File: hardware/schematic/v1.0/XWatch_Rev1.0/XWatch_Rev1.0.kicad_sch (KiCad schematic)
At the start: 0 parts

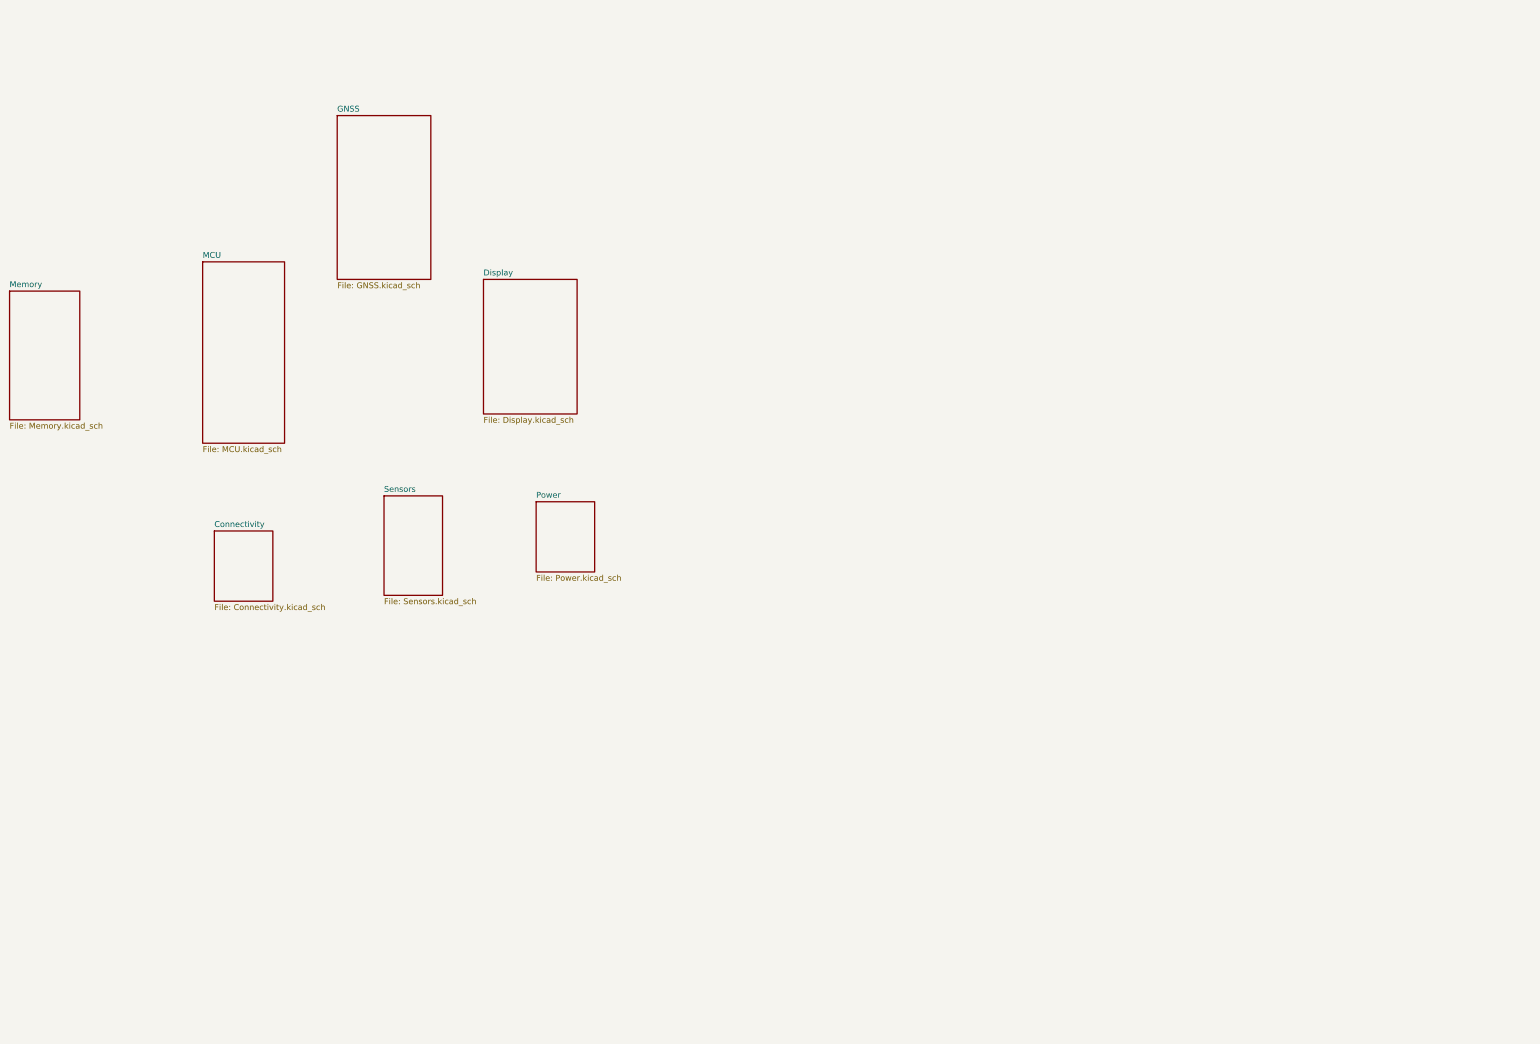
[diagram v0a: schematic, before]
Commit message: doc and sch update
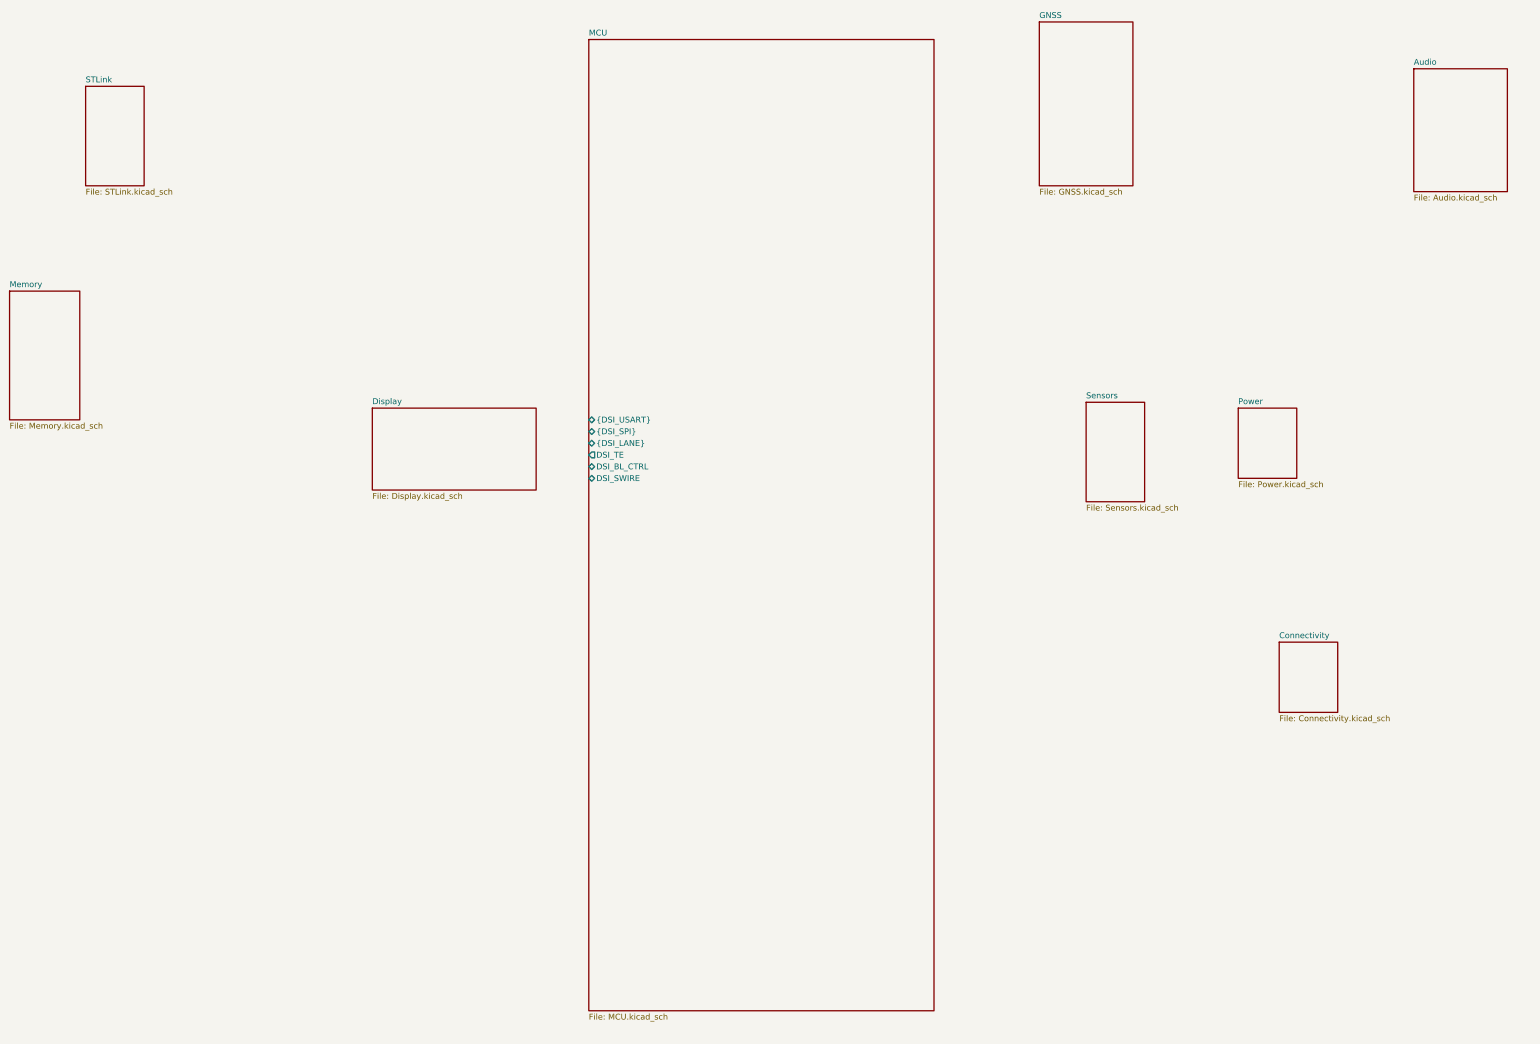
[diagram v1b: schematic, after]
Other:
- added sheet Audio (Audio.kicad_sch)
- added sheet STLink (STLink.kicad_sch)
- sheet MCU ports: added DSI_BL_CTRL, DSI_SWIRE, DSI_TE, {DSI_LANE}, {DSI_SPI}, {DSI_USART}; removed none
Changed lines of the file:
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@@
 	(generator "eeschema")
 	(generator_version "10.0")
-	(paper "A4")
+	(paper "A3")
 	(sheet
 		(at 63.5 101.6)
@@
 	)
 	(sheet
-		(at 134.62 63.5)
+		(at 287.02 43.18)
 		(size 20.32 35.56)
 		(exclude_from_sim no)
@@
 		)
 		(property "Sheetname" "GNSS"
-			(at 134.62 62.7884 0)
+			(at 287.02 42.4684 0)
 			(show_name no)
 			(do_not_autoplace no)
@@
 		)
 		(property "Sheetfile" "GNSS.kicad_sch"
-			(at 134.62 99.6446 0)
+			(at 287.02 79.3246 0)
 			(show_name no)
 			(do_not_autoplace no)
@@
 	)
 	(sheet
-		(at 144.78 146.05)
+		(at 297.18 125.73)
 		(size 12.7 21.59)
 		(exclude_from_sim no)
@@
 		)
 		(property "Sheetname" "Sensors"
-			(at 144.78 145.3384 0)
+			(at 297.18 125.0184 0)
 			(show_name no)
 			(do_not_autoplace no)
@@
 		)
 		(property "Sheetfile" "Sensors.kicad_sch"
-			(at 144.78 168.2246 0)
+			(at 297.18 147.9046 0)
 			(show_name no)
 			(do_not_autoplace no)
@@
 	)
 	(sheet
-		(at 177.8 147.32)
+		(at 330.2 127)
 		(size 12.7 15.24)
 		(exclude_from_sim no)
@@
 		)
 		(property "Sheetname" "Power"
-			(at 177.8 146.6084 0)
+			(at 330.2 126.2884 0)
 			(show_name no)
 			(do_not_autoplace no)
@@
 		)
 		(property "Sheetfile" "Power.kicad_sch"
-			(at 177.8 163.1446 0)
+			(at 330.2 142.8246 0)
 			(show_name no)
 			(do_not_autoplace no)
@@
 	)
 	(sheet
-		(at 107.95 153.67)
+		(at 339.09 177.8)
 		(size 12.7 15.24)
 		(exclude_from_sim no)
@@
 		)
 		(property "Sheetname" "Connectivity"
-			(at 107.95 152.9584 0)
+			(at 339.09 177.0884 0)
 			(show_name no)
 			(do_not_autoplace no)
@@
 		)
 		(property "Sheetfile" "Connectivity.kicad_sch"
-			(at 107.95 169.4946 0)
+			(at 339.09 193.6246 0)
 			(show_name no)
 			(do_not_autoplace no)
@@
 	)
 	(sheet
-		(at 166.37 99.06)
-		(size 20.32 29.21)
+		(at 142.24 127)
+		(size 35.56 17.78)
 		(exclude_from_sim no)
 		(in_bom yes)
@@
 		)
 		(property "Sheetname" "Display"
-			(at 166.37 98.3484 0)
+			(at 142.24 126.2884 0)
 			(show_name no)
 			(do_not_autoplace no)
@@
 		)
 		(property "Sheetfile" "Display.kicad_sch"
-			(at 166.37 128.8546 0)
+			(at 142.24 145.3646 0)
 			(show_name no)
 			(do_not_autoplace no)
@@
 	)
 	(sheet
-		(at 105.41 95.25)
-		(size 17.78 39.37)
+		(at 80.01 57.15)
+		(size 12.7 21.59)
+		(exclude_from_sim no)
+		(in_bom yes)
+		(on_board yes)
+		(dnp no)
+		(fields_autoplaced yes)
+		(stroke
+			(width 0.1524)
+			(type solid)
+		)
+		(fill
+			(color 0 0 0 0)
+		)
+		(property "Sheetname" "STLink"
+			(at 80.01 56.4384 0)
+			(show_name no)
+			(do_not_autoplace no)
+			(effects
+				(font
+					(size 1.27 1.27)
+				)
+				(justify left bottom)
+			)
+		)
+		(property "Sheetfile" "STLink.kicad_sch"
+			(at 80.01 79.3246 0)
+			(show_name no)
+			(do_not_autoplace no)
+			(effects
+				(font
+					(size 1.27 1.27)
+				)
+				(justify left top)
+			)
+		)
+		(instances
+			(project "XWatch_Rev1.0"
+				(path "/2e5e9480-7d2e-4148-a9bf-0ac7d46b20bc"
+					(page "10")
+				)
+			)
+		)
+	)
+	(sheet
+		(at 368.3 53.34)
+		(size 20.32 26.67)
+		(exclude_from_sim no)
+		(in_bom yes)
+		(on_board yes)
+		(dnp no)
+		(fields_autoplaced yes)
+		(stroke
+			(width 0.1524)
+			(type solid)
+		)
+		(fill
+			(color 0 0 0 0)
+		)
+		(property "Sheetname" "Audio"
+			(at 368.3 52.6284 0)
+			(show_name no)
+			(do_not_autoplace no)
+			(effects
+				(font
+					(size 1.27 1.27)
+				)
+				(justify left bottom)
+			)
+		)
+		(property "Sheetfile" "Audio.kicad_sch"
+			(at 368.3 80.5946 0)
+			(show_name no)
+			(do_not_autoplace no)
+			(effects
+				(font
+					(size 1.27 1.27)
+				)
+				(justify left top)
+			)
+		)
+		(instances
+			(project "XWatch_Rev1.0"
+				(path "/2e5e9480-7d2e-4148-a9bf-0ac7d46b20bc"
+					(page "9")
+				)
+			)
+		)
+	)
+	(sheet
+		(at 189.23 46.99)
+		(size 74.93 210.82)
 		(exclude_from_sim no)
 		(in_bom yes)
@@
 		)
 		(property "Sheetname" "MCU"
-			(at 105.41 94.5384 0)
+			(at 189.23 46.2784 0)
 			(show_name no)
 			(do_not_autoplace no)
@@
 		)
 		(property "Sheetfile" "MCU.kicad_sch"
-			(at 105.41 135.2046 0)
-			(show_name no)
-			(do_not_autoplace no)
-			(effects
-				(font
-					(size 1.27 1.27)
-				)
-				(justify left top)
-			)
-		)
+			(at 189.23 258.3946 0)
+			(show_name no)
+			(do_not_autoplace no)
+			(effects
+				(font
+					(size 1.27 1.27)
+				)
+				(justify left top)
+			)
+		)
+		(pin "{DSI_SPI}" bidirectional
+			(at 189.23 132.08 180)
+			(effects
+				(font
+					(size 1.27 1.27)
+				)
+				(justify left)
+			)
+		)
+		(pin "{DSI_USART}" bidirectional
+			(at 189.23 129.54 180)
+			(effects
+				(font
+					(size 1.27 1.27)
+				)
+				(justify left)
+			)
+		)
+		(pin "{DSI_LANE}" bidirectional
+			(at 189.23 134.62 180)
+			(effects
+				(font
+					(size 1.27 1.27)
+				)
+				(justify left)
+			)
+		)
+		(pin "DSI_TE" output
+			(at 189.23 137.16 180)
+			(effects
+				(font
+					(size 1.27 1.27)
+				)
+				(justify left)
+			)
+		)
+		(pin "DSI_BL_CTRL" bidirectional
+			(at 189.23 139.7 180)
+			(effects
+				(font
+					(size 1.27 1.27)
+				)
+				(justify left)
+			)
+		)
+		(pin "DSI_SWIRE" bidirectional
+			(at 189.23 142.24 180)
+			(effects
+				(font
+					(size 1.27 1.27)
+				)
+				(justify left)
+			)
+		)

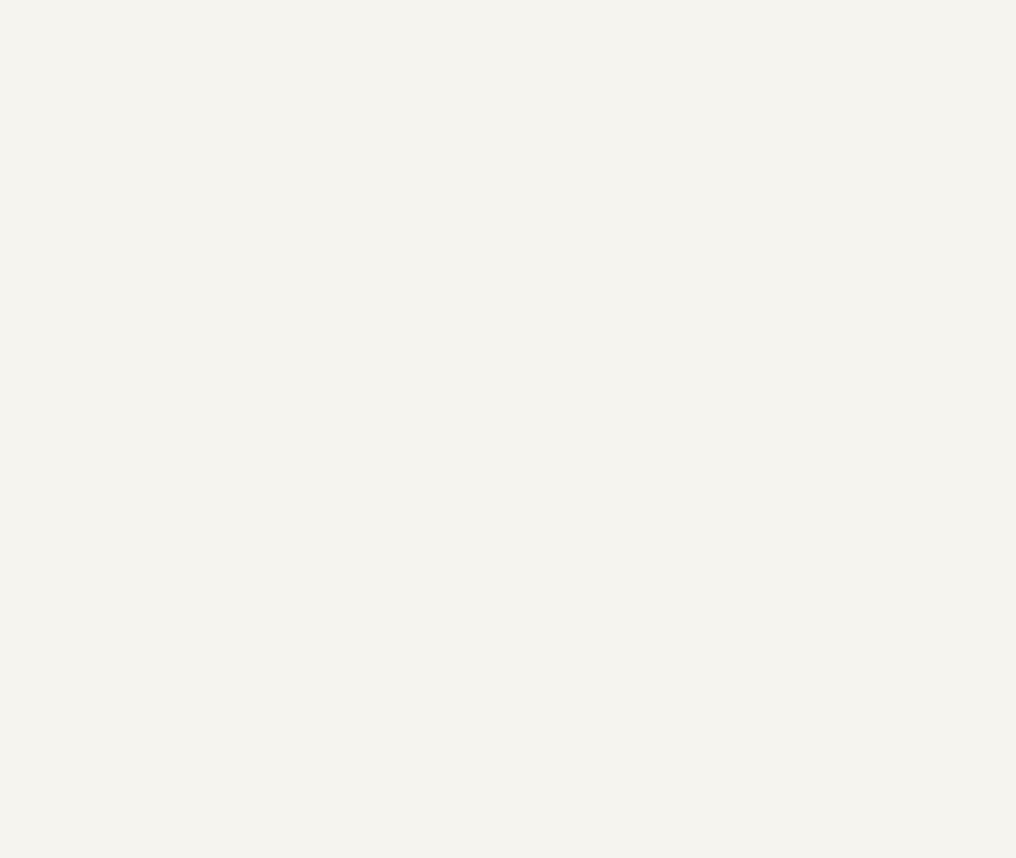
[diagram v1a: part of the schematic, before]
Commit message: doc and sch update
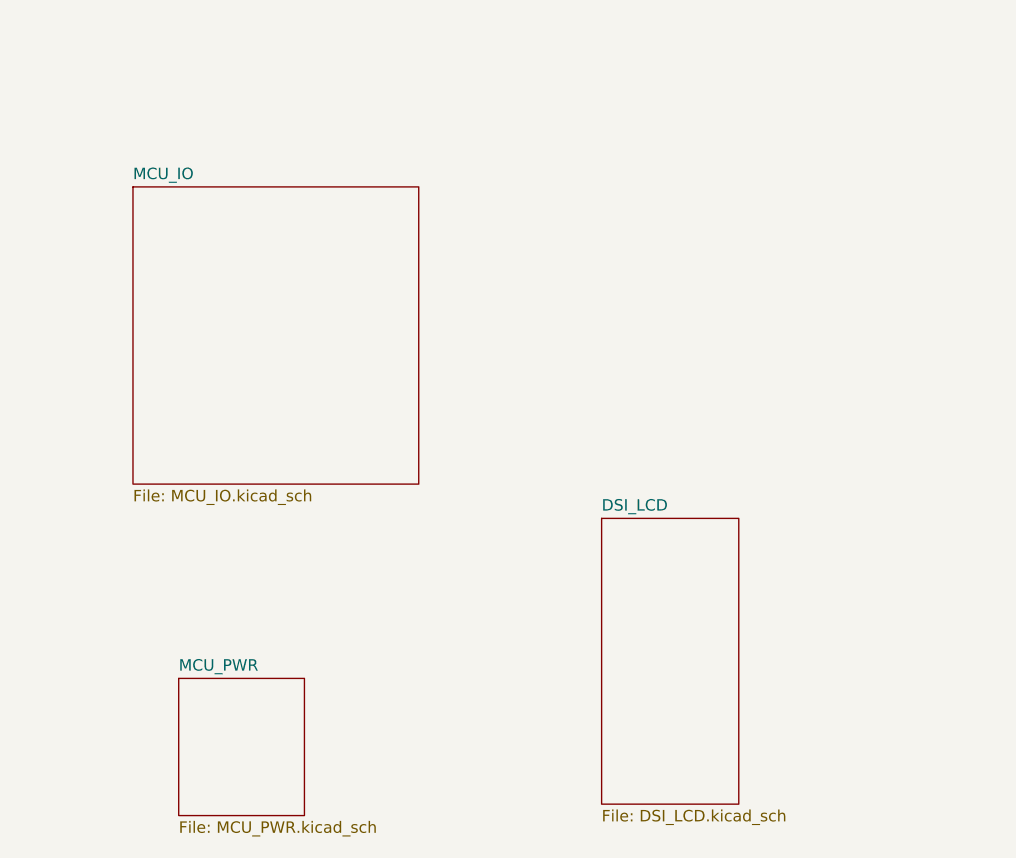
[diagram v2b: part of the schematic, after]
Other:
- added sheet DSI_LCD (DSI_LCD.kicad_sch)
- added sheet MCU_IO (MCU_IO.kicad_sch)
- added sheet MCU_PWR (MCU_PWR.kicad_sch)
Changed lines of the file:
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@@
+	)
+	(sheet
+		(at 81.28 245.11)
+		(size 13.97 15.24)
+		(exclude_from_sim no)
+		(in_bom yes)
+		(on_board yes)
+		(dnp no)
+		(fields_autoplaced yes)
+		(stroke
+			(width 0.1524)
+			(type solid)
+		)
+		(fill
+			(color 0 0 0 0)
+		)
+		(property "Sheetname" "MCU_PWR"
+			(at 81.28 244.3984 0)
+			(show_name no)
+			(do_not_autoplace no)
+			(effects
+				(font
+					(size 1.27 1.27)
+				)
+				(justify left bottom)
+			)
+		)
+		(property "Sheetfile" "MCU_PWR.kicad_sch"
+			(at 81.28 260.9346 0)
+			(show_name no)
+			(do_not_autoplace no)
+			(effects
+				(font
+					(size 1.27 1.27)
+				)
+				(justify left top)
+			)
+		)
+		(instances
+			(project "XWatch_Rev1.0"
+				(path "/2e5e9480-7d2e-4148-a9bf-0ac7d46b20bc"
+					(page "13")
+				)
+			)
+		)
+	)
+	(sheet
+		(at 128.27 227.33)
+		(size 15.24 31.75)
+		(exclude_from_sim no)
+		(in_bom yes)
+		(on_board yes)
+		(dnp no)
+		(fields_autoplaced yes)
+		(stroke
+			(width 0.1524)
+			(type solid)
+		)
+		(fill
+			(color 0 0 0 0)
+		)
+		(property "Sheetname" "DSI_LCD"
+			(at 128.27 226.6184 0)
+			(show_name no)
+			(do_not_autoplace no)
+			(effects
+				(font
+					(size 1.27 1.27)
+				)
+				(justify left bottom)
+			)
+		)
+		(property "Sheetfile" "DSI_LCD.kicad_sch"
+			(at 128.27 259.6646 0)
+			(show_name no)
+			(do_not_autoplace no)
+			(effects
+				(font
+					(size 1.27 1.27)
+				)
+				(justify left top)
+			)
+		)
+		(instances
+			(project "XWatch_Rev1.0"
+				(path "/2e5e9480-7d2e-4148-a9bf-0ac7d46b20bc"
+					(page "12")
+				)
+			)
+		)
 	)
 	(sheet
@@
 				)
 			)
+		)
+	)
+	(sheet
+		(at 76.2 190.5)
+		(size 31.75 33.02)
+		(exclude_from_sim no)
+		(in_bom yes)
+		(on_board yes)
+		(dnp no)
+		(fields_autoplaced yes)
+		(stroke
+			(width 0.1524)
+			(type solid)
+		)
+		(fill
+			(color 0 0 0 0)
+		)
+		(property "Sheetname" "MCU_IO"
+			(at 76.2 189.7884 0)
+			(show_name no)
+			(do_not_autoplace no)
+			(effects
+				(font
+					(size 1.27 1.27)
+				)
+				(justify left bottom)
+			)
+		)
+		(property "Sheetfile" "MCU_IO.kicad_sch"
+			(at 76.2 224.1046 0)
+			(show_name no)
+			(do_not_autoplace no)
+			(effects
+				(font
+					(size 1.27 1.27)
+				)
+				(justify left top)
+			)
+		)
+		(instances
+			(project "XWatch_Rev1.0"
+				(path "/2e5e9480-7d2e-4148-a9bf-0ac7d46b20bc"
+					(page "11")
+				)
+			)

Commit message: add rev2.0
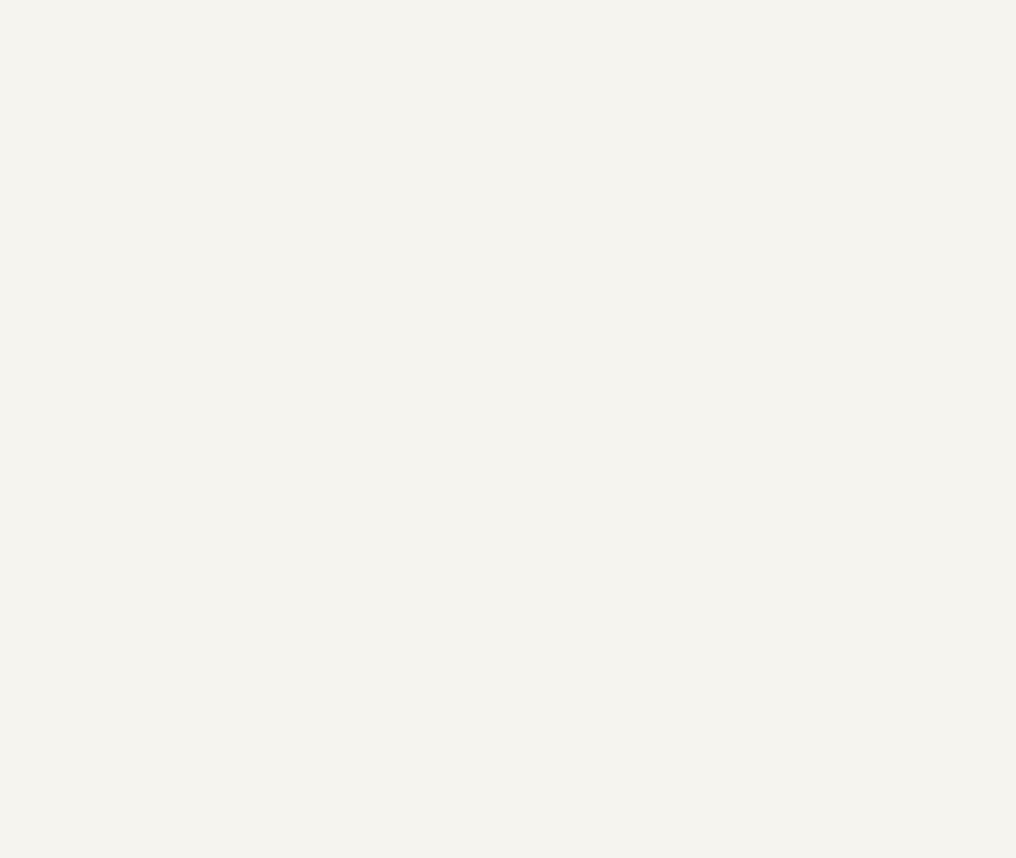
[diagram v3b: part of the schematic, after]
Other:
- removed sheet DSI_LCD
- removed sheet MCU_IO
- removed sheet MCU_PWR
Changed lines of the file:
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@@
-	)
-	(sheet
-		(at 81.28 245.11)
-		(size 13.97 15.24)
-		(exclude_from_sim no)
-		(in_bom yes)
-		(on_board yes)
-		(dnp no)
-		(fields_autoplaced yes)
-		(stroke
-			(width 0.1524)
-			(type solid)
-		)
-		(fill
-			(color 0 0 0 0)
-		)
-		(property "Sheetname" "MCU_PWR"
-			(at 81.28 244.3984 0)
-			(show_name no)
-			(do_not_autoplace no)
-			(effects
-				(font
-					(size 1.27 1.27)
-				)
-				(justify left bottom)
-			)
-		)
-		(property "Sheetfile" "MCU_PWR.kicad_sch"
-			(at 81.28 260.9346 0)
-			(show_name no)
-			(do_not_autoplace no)
-			(effects
-				(font
-					(size 1.27 1.27)
-				)
-				(justify left top)
-			)
-		)
-		(instances
-			(project "XWatch_Rev1.0"
-				(path "/2e5e9480-7d2e-4148-a9bf-0ac7d46b20bc"
-					(page "13")
-				)
-			)
-		)
-	)
-	(sheet
-		(at 128.27 227.33)
-		(size 15.24 31.75)
-		(exclude_from_sim no)
-		(in_bom yes)
-		(on_board yes)
-		(dnp no)
-		(fields_autoplaced yes)
-		(stroke
-			(width 0.1524)
-			(type solid)
-		)
-		(fill
-			(color 0 0 0 0)
-		)
-		(property "Sheetname" "DSI_LCD"
-			(at 128.27 226.6184 0)
-			(show_name no)
-			(do_not_autoplace no)
-			(effects
-				(font
-					(size 1.27 1.27)
-				)
-				(justify left bottom)
-			)
-		)
-		(property "Sheetfile" "DSI_LCD.kicad_sch"
-			(at 128.27 259.6646 0)
-			(show_name no)
-			(do_not_autoplace no)
-			(effects
-				(font
-					(size 1.27 1.27)
-				)
-				(justify left top)
-			)
-		)
-		(instances
-			(project "XWatch_Rev1.0"
-				(path "/2e5e9480-7d2e-4148-a9bf-0ac7d46b20bc"
-					(page "12")
-				)
-			)
-		)
 	)
 	(sheet
@@
 				)
 			)
-		)
-	)
-	(sheet
-		(at 76.2 190.5)
-		(size 31.75 33.02)
-		(exclude_from_sim no)
-		(in_bom yes)
-		(on_board yes)
-		(dnp no)
-		(fields_autoplaced yes)
-		(stroke
-			(width 0.1524)
-			(type solid)
-		)
-		(fill
-			(color 0 0 0 0)
-		)
-		(property "Sheetname" "MCU_IO"
-			(at 76.2 189.7884 0)
-			(show_name no)
-			(do_not_autoplace no)
-			(effects
-				(font
-					(size 1.27 1.27)
-				)
-				(justify left bottom)
-			)
-		)
-		(property "Sheetfile" "MCU_IO.kicad_sch"
-			(at 76.2 224.1046 0)
-			(show_name no)
-			(do_not_autoplace no)
-			(effects
-				(font
-					(size 1.27 1.27)
-				)
-				(justify left top)
-			)
-		)
-		(instances
-			(project "XWatch_Rev1.0"
-				(path "/2e5e9480-7d2e-4148-a9bf-0ac7d46b20bc"
-					(page "11")
-				)
-			)
